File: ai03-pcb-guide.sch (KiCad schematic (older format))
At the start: 24 parts, among them SW1 SW_Push, U1 ATmega32U4-AU, Y1 16MHz

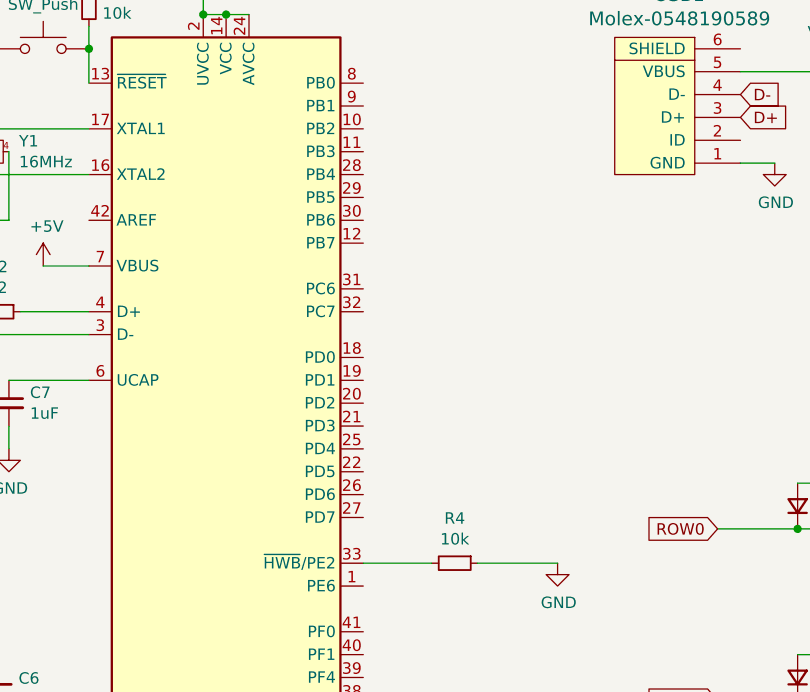
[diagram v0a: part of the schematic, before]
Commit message: Route to switches
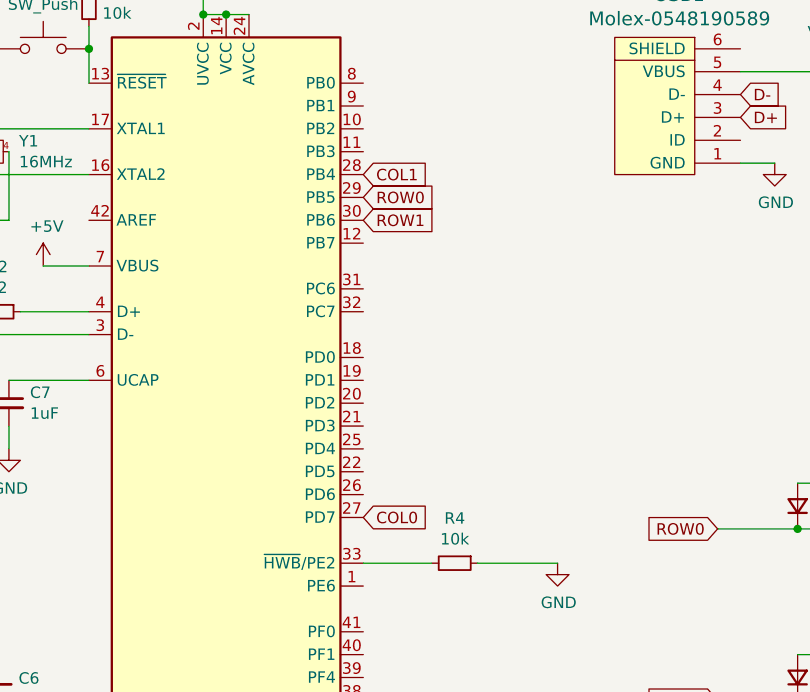
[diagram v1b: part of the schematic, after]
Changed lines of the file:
@@
 Text GLabel 5650 5000 0    50   Input ~ 0
 ROW1
+Text GLabel 4100 2700 2    50   Input ~ 0
+COL1
+Text GLabel 4100 2800 2    50   Input ~ 0
+ROW0
+Text GLabel 4100 2900 2    50   Input ~ 0
+ROW1
+Text GLabel 4100 4200 2    50   Input ~ 0
+COL0
 $EndSCHEMATC
